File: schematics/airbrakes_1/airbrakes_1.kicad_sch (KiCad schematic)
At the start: 7 parts, among them U6 XL1509-3.3

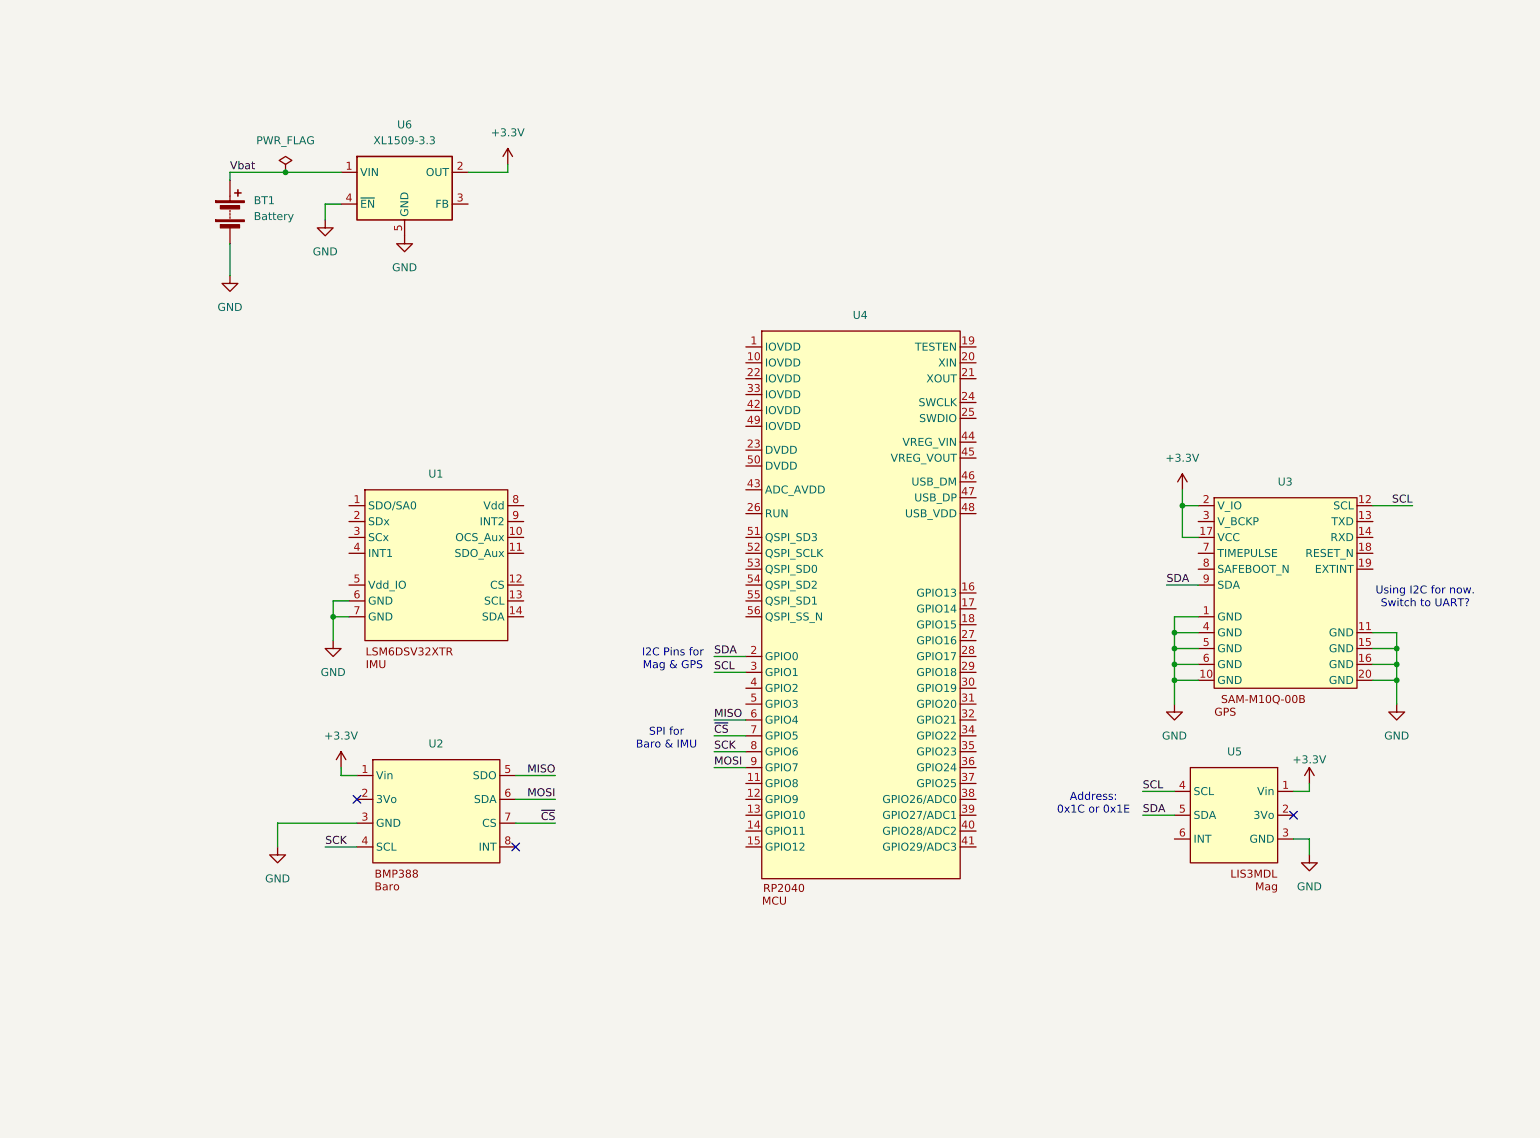
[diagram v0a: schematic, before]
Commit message: Finish communication routing, organize into sections
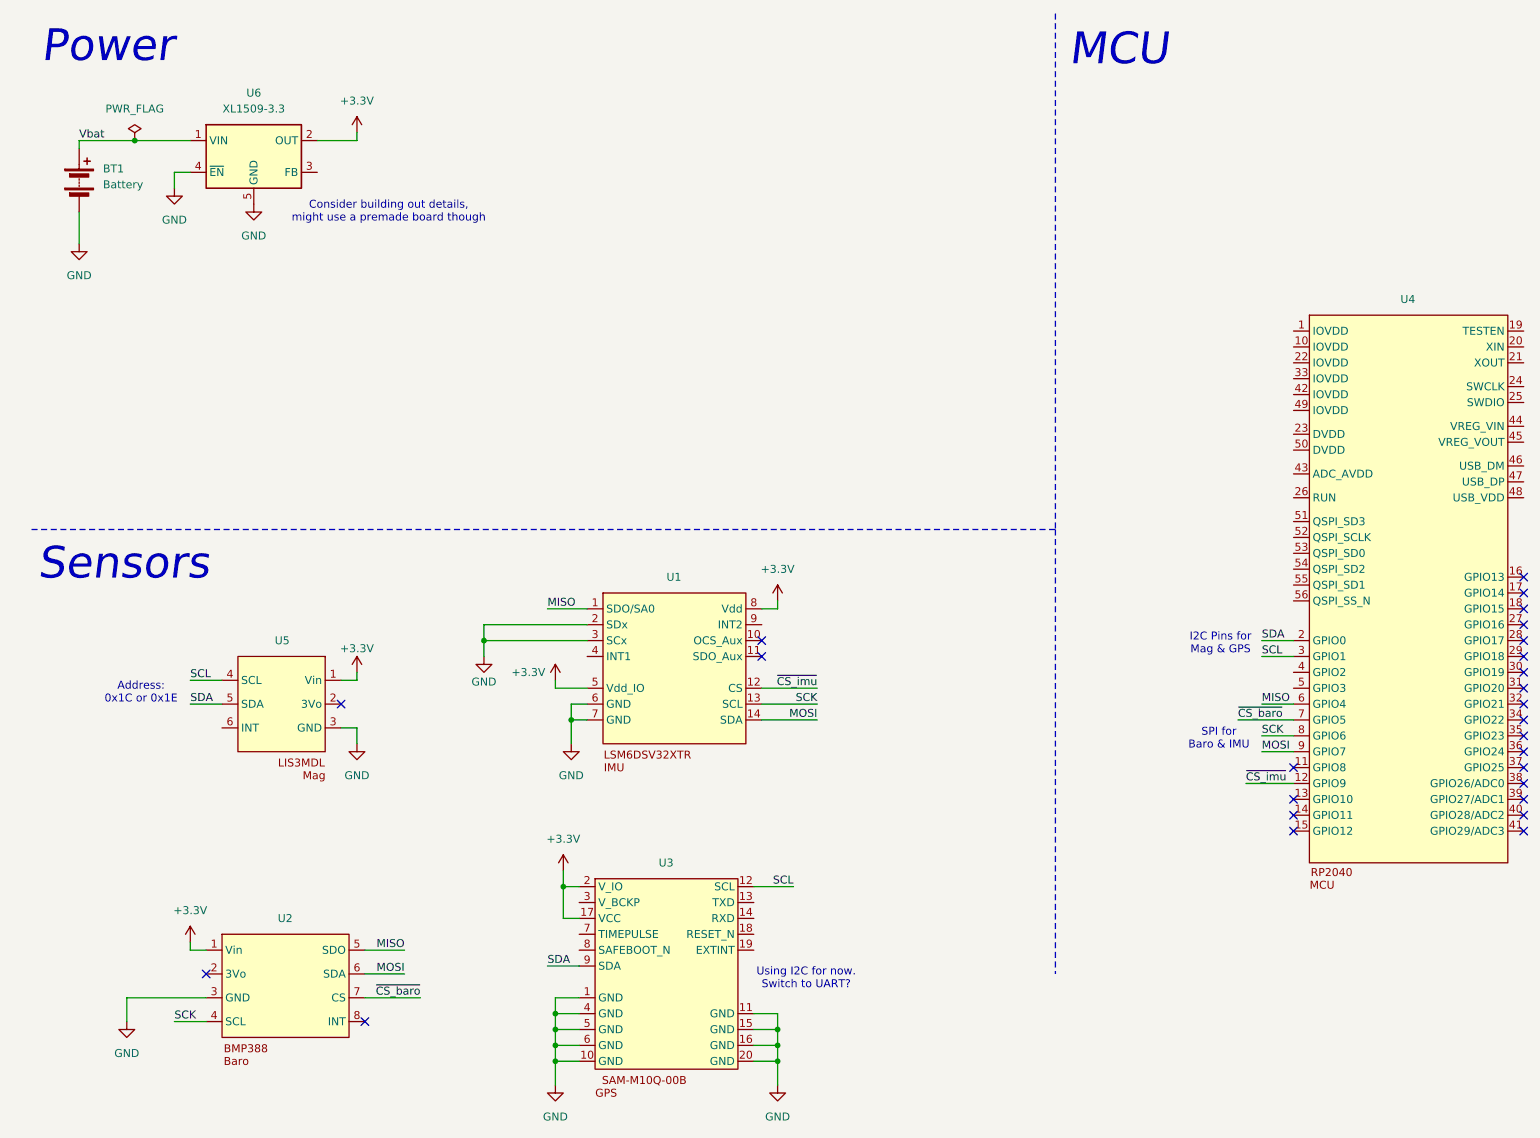
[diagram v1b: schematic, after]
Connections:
- net +3.3V: now also U1.5 (Vdd_IO), U1.8 (Vdd)
- net GND: now also U1.2 (SDx), U1.3 (SCx)
- net MISO: now also U1.1 (SDO/SA0)
- net MOSI: now also U1.14 (SDA)
- net SCK: now also U1.13 (SCL)
- net ~{CS_imu}: now reaches U1.12 (CS)
- net ~{CS_imu}: now also U4.12 (GPIO9)
- net ~{CS} renamed ~{CS_baro}
- no-connect marks 3 -> 26
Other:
- note added: "Consider building out details, might use a premade board though"
- note added: "MCU"
- note added: "Power"
- note added: "Sensors"
- moved on the sheet: BT1, U1, U2, U3, U4, U5, U6
